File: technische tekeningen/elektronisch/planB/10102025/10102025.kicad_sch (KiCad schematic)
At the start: 7 parts, among them M1 Motor_DC, M2 Motor_DC, SW1 Start

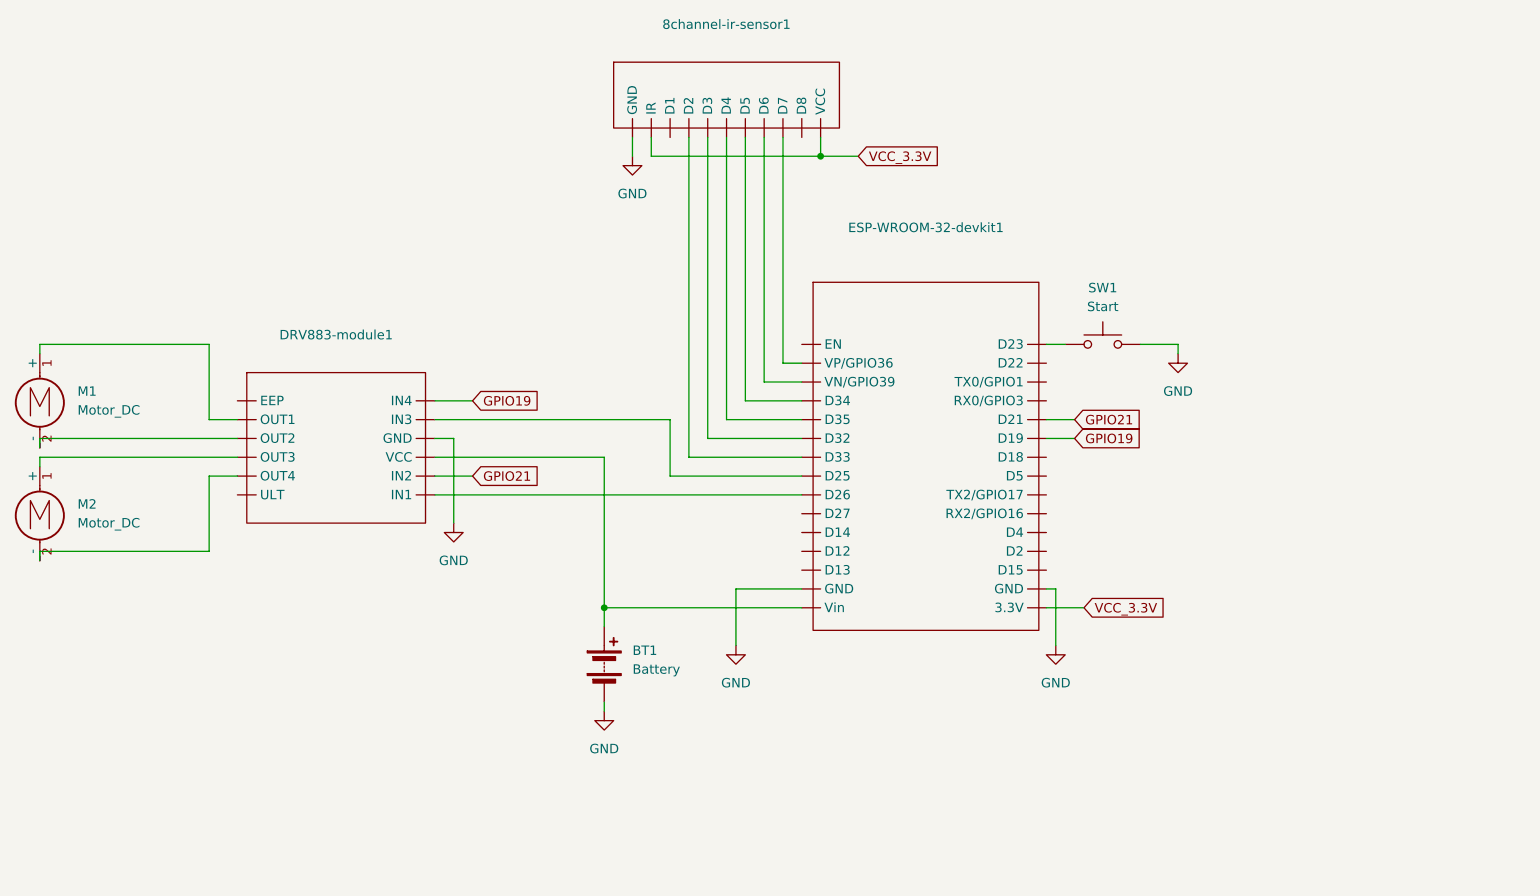
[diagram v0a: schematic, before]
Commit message: com
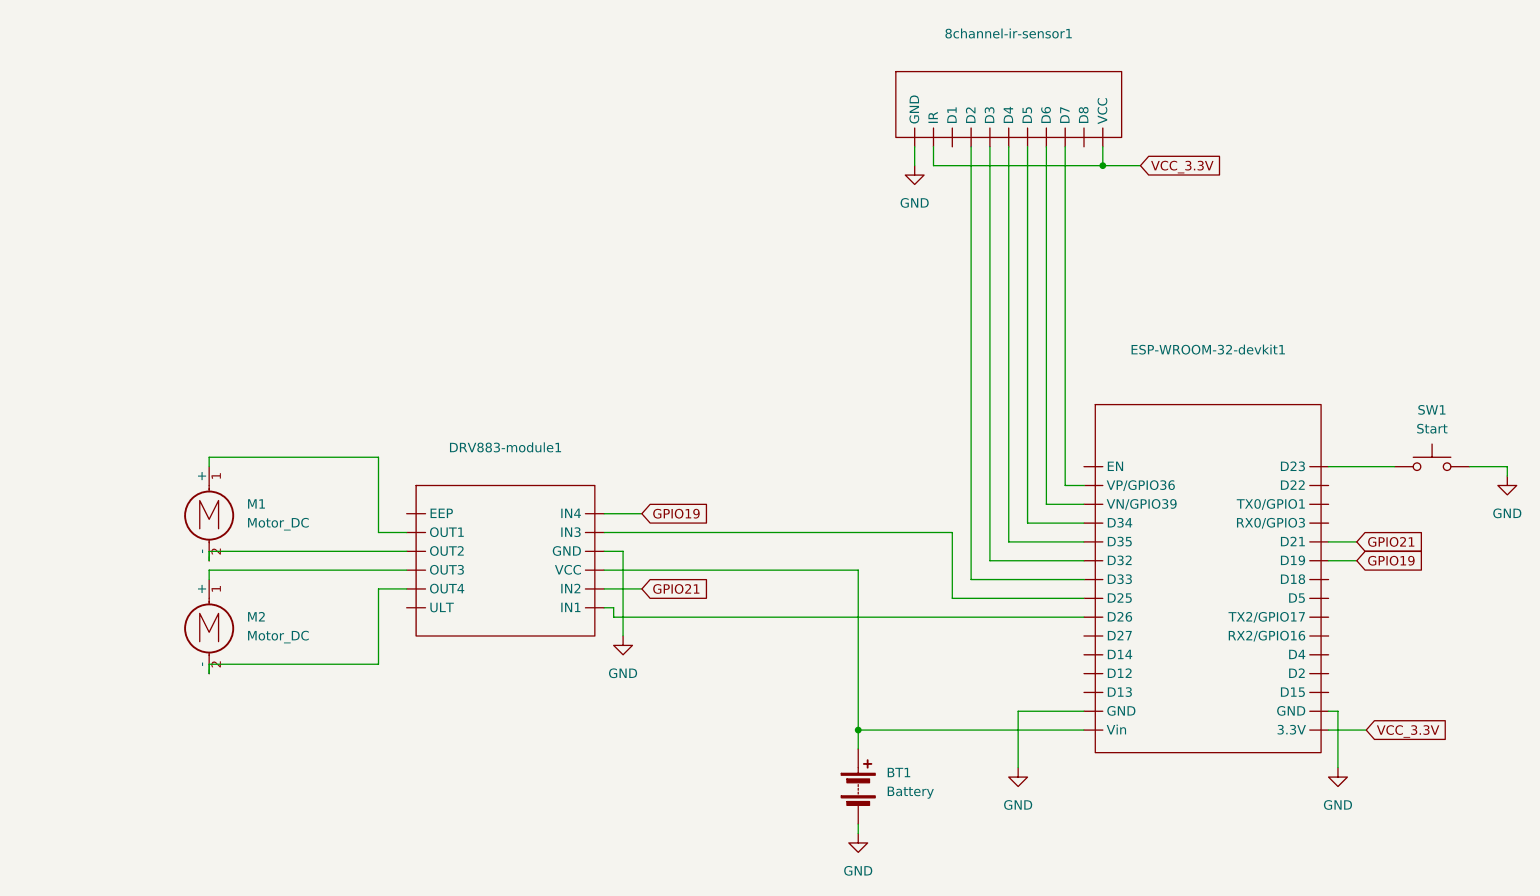
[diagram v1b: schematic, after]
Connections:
- new net: 8channel-ir-sensor1. (VCC), ESP-WROOM-32-devkit1. (3.3V) (x6)
- new net: BT1.1 (+), DRV883-module1. (IN1), ESP-WROOM-32-devkit1. (3.3V)
- new net: DRV883-module1. (IN1), ESP-WROOM-32-devkit1. (3.3V) (x2)
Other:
- moved on the sheet: 8channel-ir-sensor1, BT1, DRV883-module1, ESP-WROOM-32-devkit1, M1, M2, SW1
